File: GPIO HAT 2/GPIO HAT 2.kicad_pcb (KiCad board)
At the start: 4 copper layers, 85 x 74.6 mm, 106 parts, among them J1 ., J10 ., J11 ., J12 ., J13 ., J14 ., J15 ., J16 ., J17 ., J18 ., J19 ., J2 ., J20 ., J21 LVDS, J22 LVDS, J23 USB_C_Receptacle_PowerOnly_6P, J24 02x02, J3 ., J4 ., J5 ., J6 ., J7 ., J8 ., J9 ., U1 TXB0108DQSR, U10 TXB0108DQSR, U11 SY8088IAAC, U12 SY8088IAAC, U13 TPS2117, U2 TXB0108DQSR, U3 TXB0108DQSR, U4 TXB0108DQSR, U5 TXB0108DQSR, U6 TXB0108DQSR, U7 TXB0108DQSR, U8 TXB0108DQSR, U9 TXB0108DQSR

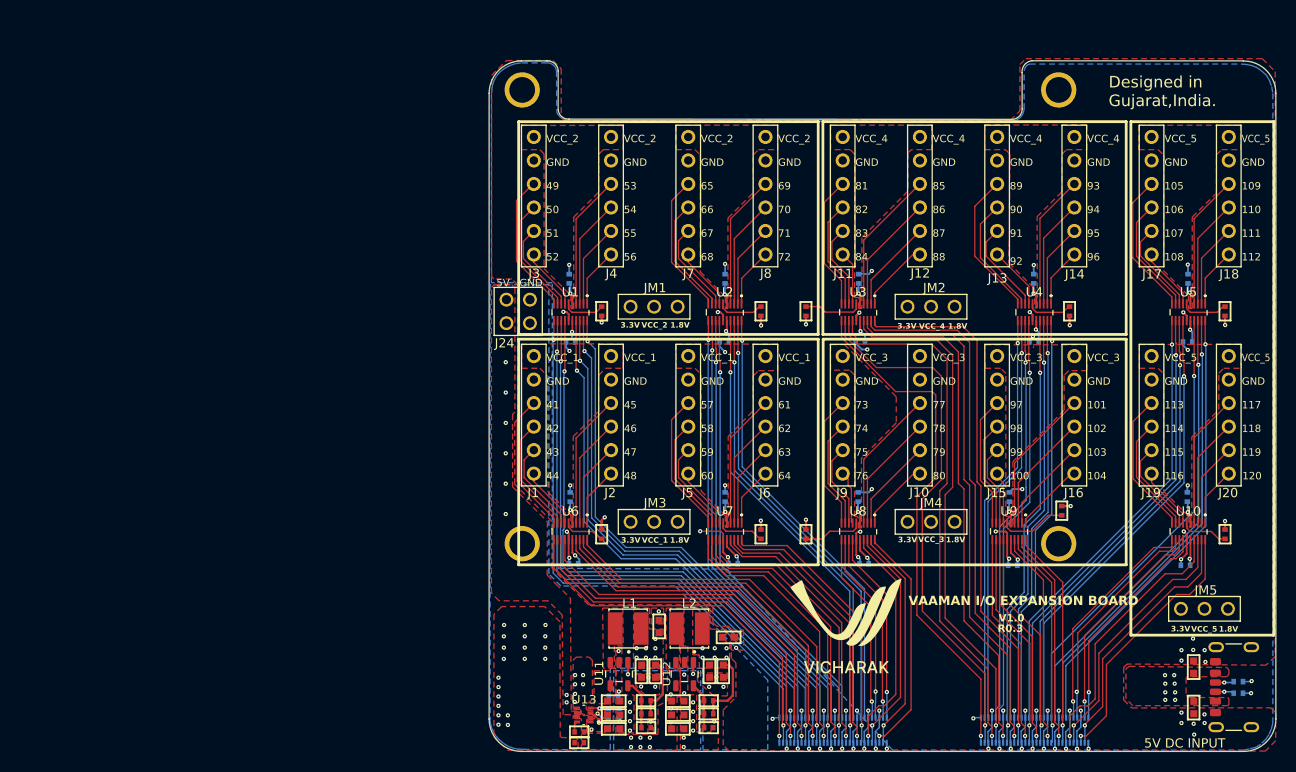
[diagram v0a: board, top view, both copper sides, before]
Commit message: Project file generated
BOM, HTML , PDFs
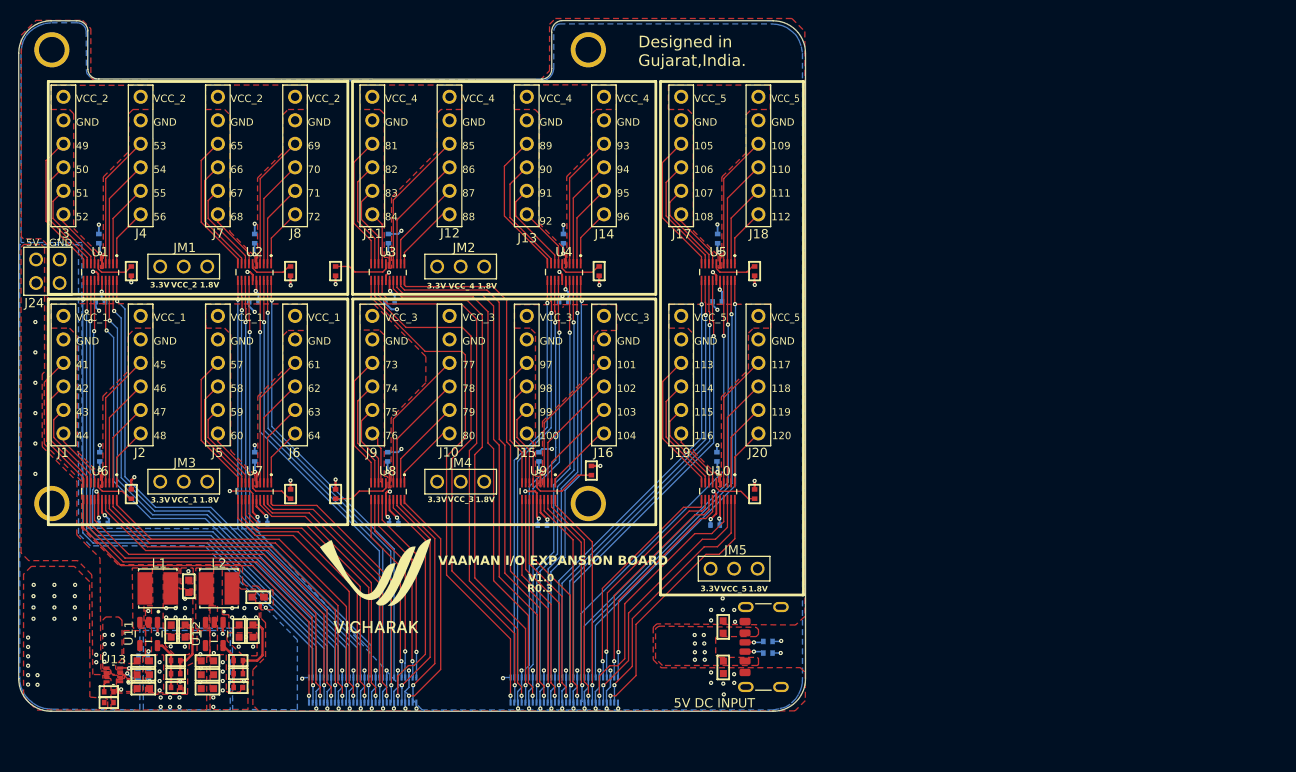
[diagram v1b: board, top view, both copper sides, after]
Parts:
- C10, C11, C19, C20, C21, C23, C24, C25, C26, C27, C28, C29, C30, C31, C32, C33, C34, C35, C36, C37, C38: value 0.1uF -> 100nF
- C22: value 0.1uF -> 100nf
- R2: value 22.2K -> 22.1K
- moved C10 51.0 mm to (114.7, 131.3)
- moved C15 51.0 mm to (128.7, 126.8)
- moved C16 51.0 mm to (130.3, 123.6)
- moved C17 51.0 mm to (128.8, 123.6)
- moved C18 51.0 mm to (130.9, 119.9)
- moved C19 51.0 mm to (113.7, 104.8)
- moved C20 51.0 mm to (113.6, 81.3)
- moved C22 51.0 mm to (144.9, 81.3)
- moved C24 51.0 mm to (161.2, 104.8)
- moved C30 51.0 mm to (161.6, 112.2)
- moved C32 51.0 mm to (144.8, 104.8)
- moved C35 51.0 mm to (130.4, 88.1)
- moved C36 51.0 mm to (145.5, 112.1)
- moved C4 51.0 mm to (122.0, 126.8)
- moved C6 51.0 mm to (121.5, 123.6)
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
